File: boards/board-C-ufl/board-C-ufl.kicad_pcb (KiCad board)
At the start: 4 copper layers, 69.7 x 99 mm, 30 parts, among them J5 SAMTEC_QSE-040-01-X-D-A, K0 U.FL_Hirose_U.FL-R-SMT-1_Vert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, K1 U.FL_Hirose_U.FL-R-SMT-1_Vert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, K10 U.FL_Hirose_U.FL-R-SMT-1_Vert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, K11 U.FL_Hirose_U.FL-R-SMT-1_Vert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, K12 U.FL_Hirose_U.FL-R-SMT-1_Vert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, K13 U.FL_Hirose_U.FL-R-SMT-1_Vert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, K14 U.FL_Hirose_U.FL-R-SMT-1_Vert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, K15 U.FL_Hirose_U.FL-R-SMT-1_Vert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, K16 U.FL_Hirose_U.FL-R-SMT-1_Vert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, K17 U.FL_Hirose_U.FL-R-SMT-1_Vert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, K18 U.FL_Hirose_U.FL-R-SMT-1_Vert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, K19 U.FL_Hirose_U.FL-R-SMT-1_Vert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, K2 U.FL_Hirose_U.FL-R-SMT-1_Vert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, K20 U.FL_Hirose_U.FL-R-SMT-1_Vert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, K21 U.FL_Hirose_U.FL-R-SMT-1_Vert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, K22 U.FL_Hirose_U.FL-R-SMT-1_Vert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, K23 U.FL_Hirose_U.FL-R-SMT-1_Vert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, K3 U.FL_Hirose_U.FL-R-SMT-1_Vert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, K4 U.FL_Hirose_U.FL-R-SMT-1_Vert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, K5 U.FL_Hirose_U.FL-R-SMT-1_Vert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, K6 U.FL_Hirose_U.FL-R-SMT-1_Vert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, K7 U.FL_Hirose_U.FL-R-SMT-1_Vert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, K8 U.FL_Hirose_U.FL-R-SMT-1_Vert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, K9 U.FL_Hirose_U.FL-R-SMT-1_Vert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

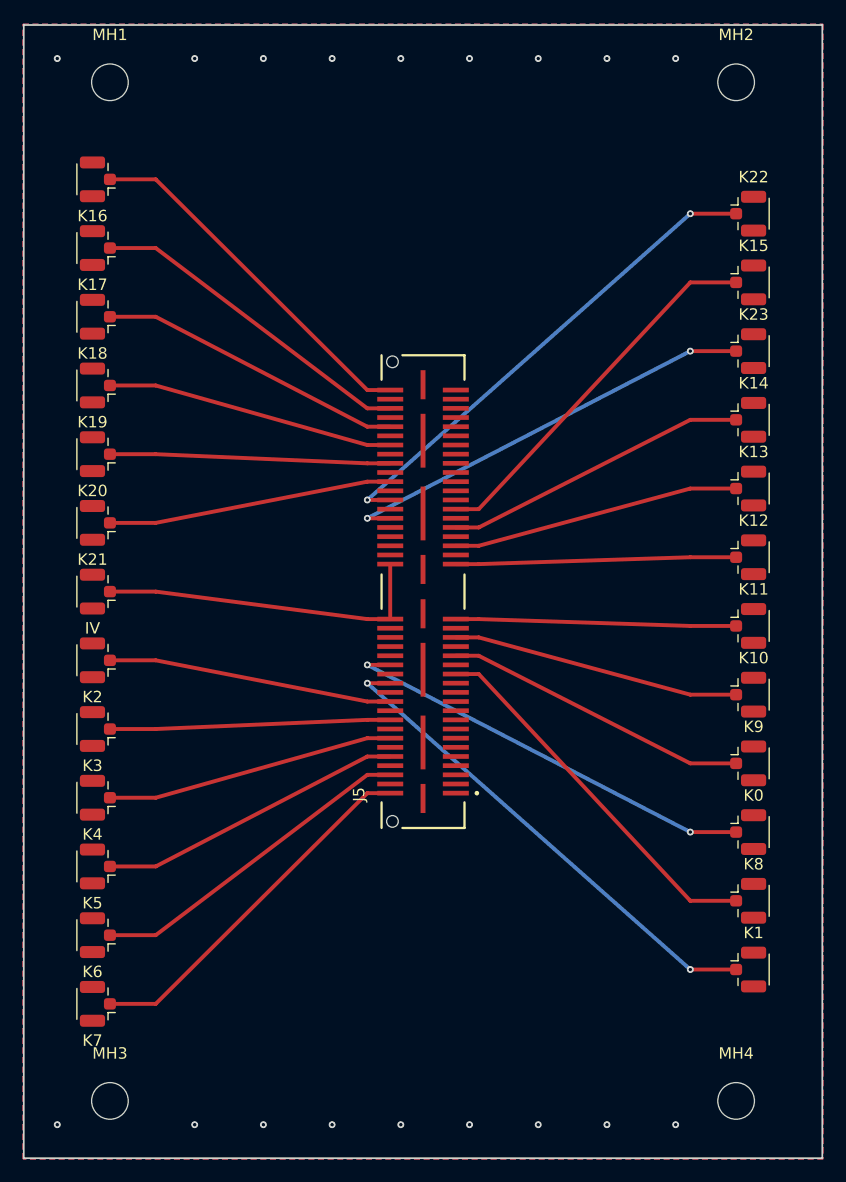
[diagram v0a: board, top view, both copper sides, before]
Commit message: initial upload
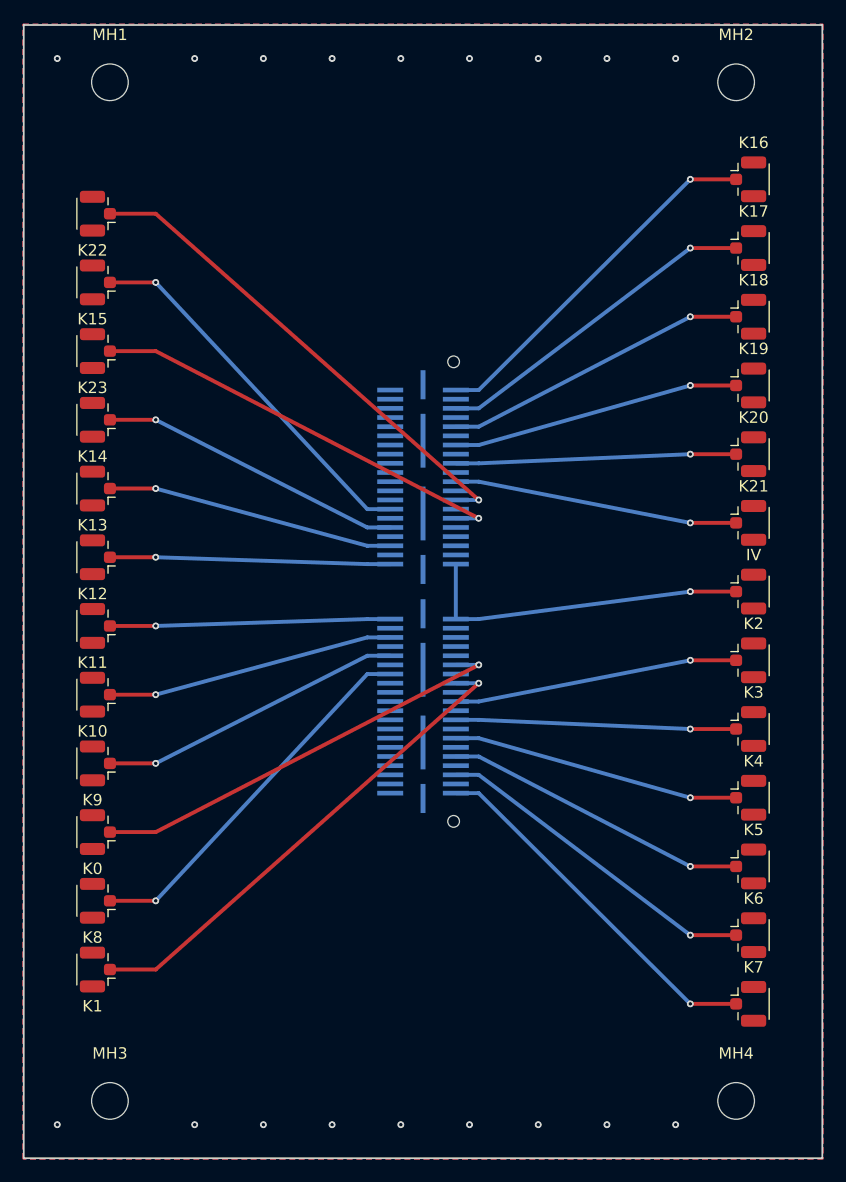
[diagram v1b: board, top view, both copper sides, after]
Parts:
- J5: moved to B.Cu
- moved IV 57.7 mm to (72.7, 59.5), turned to 0 degrees
- moved K0 57.7 mm to (15.0, 80.5), turned to 180 degrees
- moved K1 57.7 mm to (15.0, 92.5), turned to 180 degrees
- moved K10 57.7 mm to (15.0, 68.5), turned to 180 degrees
- moved K11 57.7 mm to (15.0, 62.5), turned to 180 degrees
- moved K12 57.7 mm to (15.0, 56.5), turned to 180 degrees
- moved K13 57.7 mm to (15.0, 50.5), turned to 180 degrees
- moved K14 57.7 mm to (15.0, 44.5), turned to 180 degrees
- moved K15 57.7 mm to (15.0, 32.5), turned to 180 degrees
- moved K16 57.7 mm to (72.7, 23.5), turned to 0 degrees
- moved K17 57.7 mm to (72.7, 29.5), turned to 0 degrees
- moved K18 57.7 mm to (72.7, 35.5), turned to 0 degrees
- moved K19 57.7 mm to (72.7, 41.5), turned to 0 degrees
- moved K2 57.7 mm to (72.7, 65.5), turned to 0 degrees
- moved K20 57.7 mm to (72.7, 47.5), turned to 0 degrees
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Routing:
- net SIPM_K9: vias 0 -> 1
- net SIPM_K8: vias 0 -> 1
- net SIPM_K7: vias 0 -> 1
- net SIPM_K6: vias 0 -> 1
- net SIPM_K5: vias 0 -> 1
- net SIPM_K4: vias 0 -> 1
- net SIPM_K3: vias 0 -> 1
- net SIPM_K23: vias 2 -> 1
- net SIPM_K22: vias 2 -> 1
- net SIPM_K21: vias 0 -> 1
- net SIPM_K20: vias 0 -> 1
- net SIPM_K2: vias 0 -> 1
- net SIPM_K19: vias 0 -> 1
- net SIPM_K18: vias 0 -> 1
- net SIPM_K17: vias 0 -> 1
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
